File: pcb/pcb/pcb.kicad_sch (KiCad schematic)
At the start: 12 parts, among them J1 SD Card, J2 Mic, J3 Relay Solenoid, J4 Status LED, SW1 Button Up, SW2 Button Down, SW3 Button Record, SW4 Button Delete, SW5 Button Play, U1 ESP32-C3-DevKitC-02

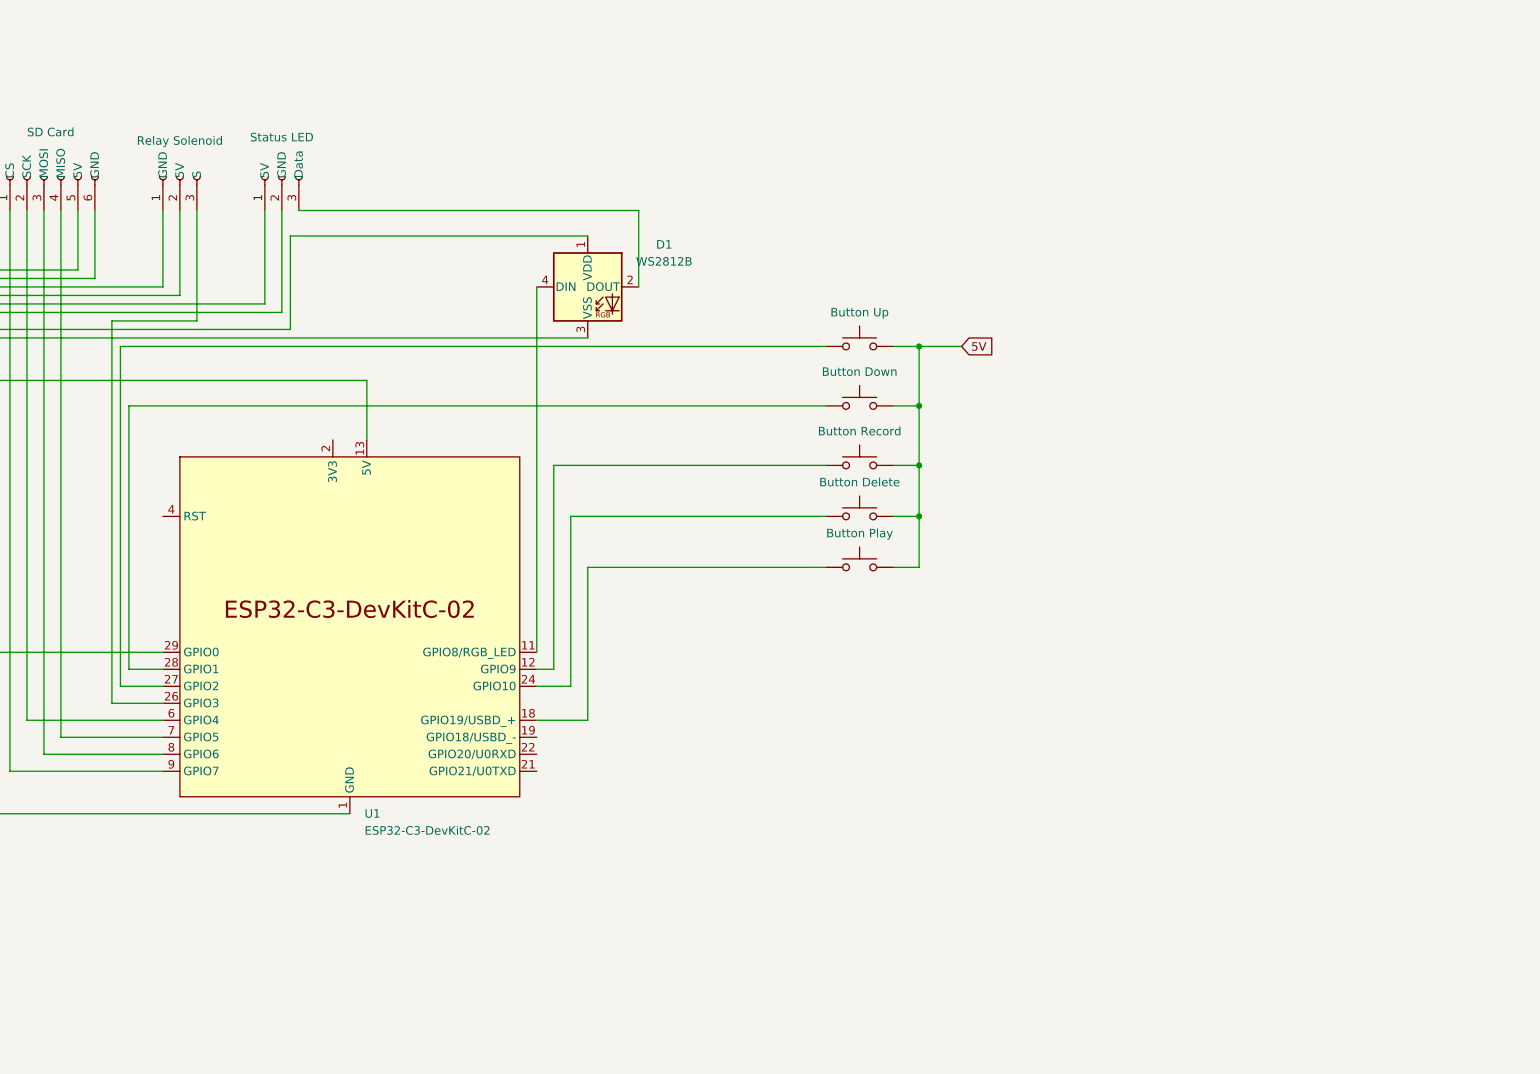
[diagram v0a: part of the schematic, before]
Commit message: update
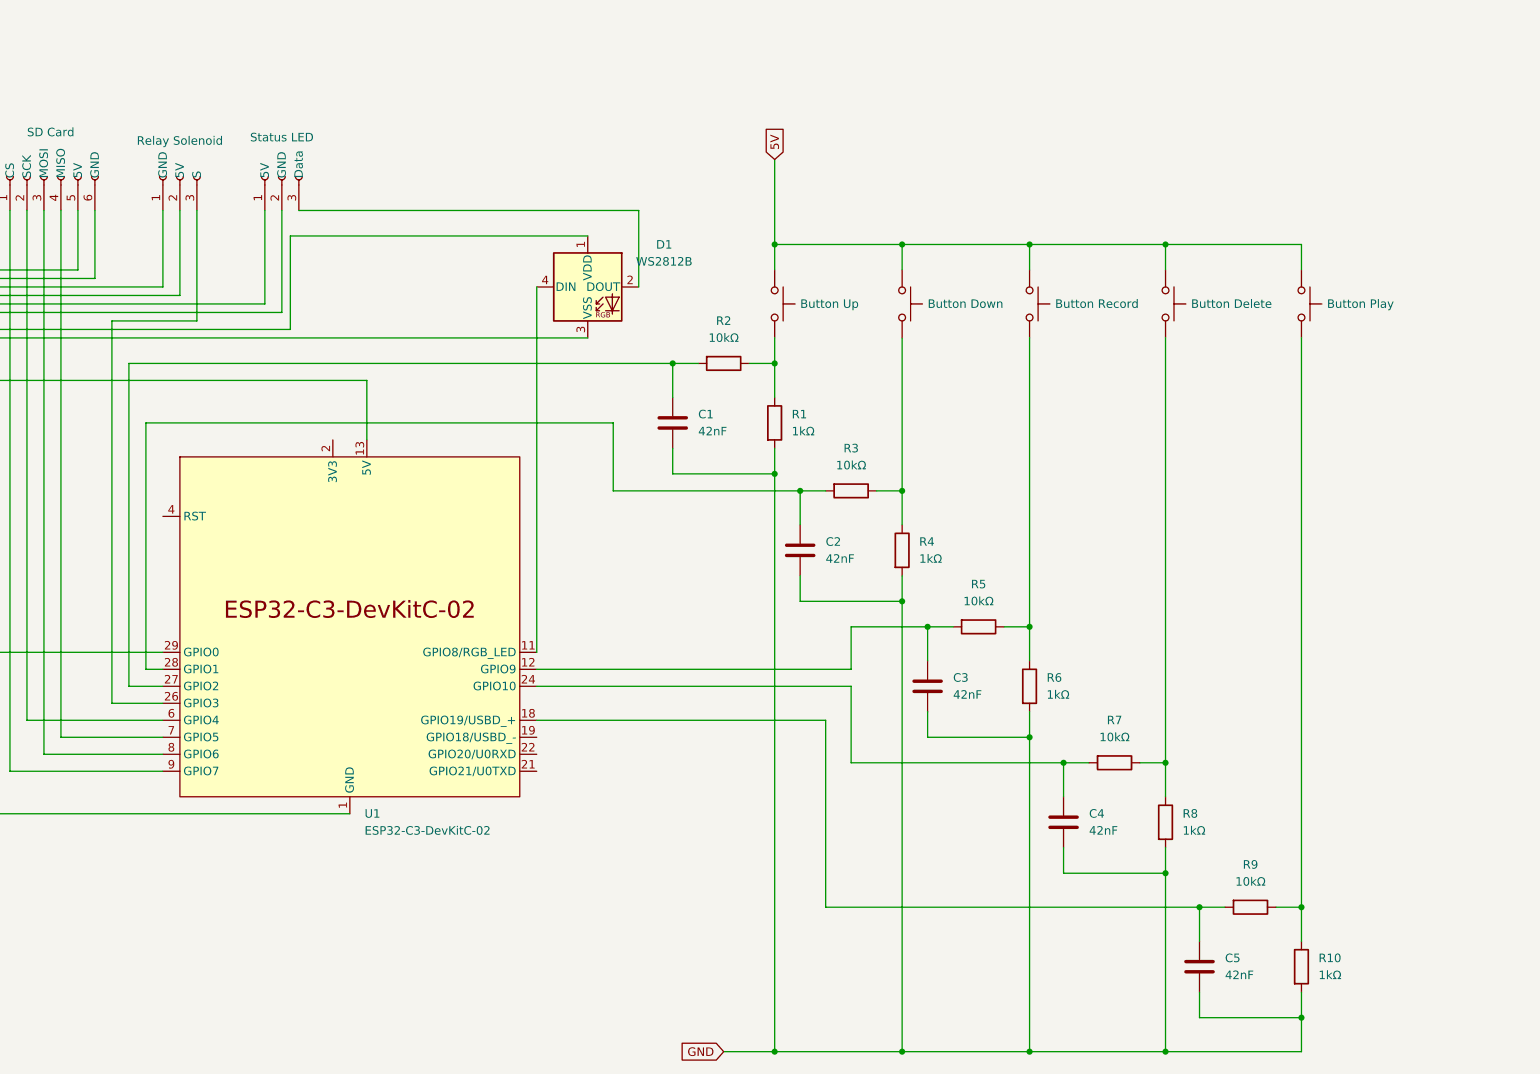
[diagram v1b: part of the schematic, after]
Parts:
- added C1, C2, C3, C4, C5: 42nF, symbol Device:C
- added R1, R10, R4, R6, R8: 1kΩ, symbol Device:R
- added R2, R3, R5, R7, R9: 10kΩ, symbol Device:R
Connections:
- net 5V: now also SW1.1, SW2.1, SW3.1, SW4.1, SW5.1; no longer SW1.2, SW2.2, SW3.2, SW4.2, SW5.2
- net GND: now also C1.2, C2.2, C3.2, C4.2, C5.2, R1.2, R10.2, R4.2, R6.2, R8.2
- net at U1.12 (GPIO9): now also C3.1, R5.2; no longer SW3.1
- net at U1.18 (GPIO19/USBD_+): now also C5.1, R9.2; no longer SW5.1
- net at U1.24 (GPIO10): now also C4.1, R7.2; no longer SW4.1
- net at U1.27 (GPIO2): now also C1.1, R2.2; no longer SW1.1
- net at U1.28 (GPIO1): now also C2.1, R3.2; no longer SW2.1
- new net: R7.1, R8.1, SW4.2
- new net: R1.1, R2.1, SW1.2
- new net: R10.1, R9.1, SW5.2
- new net: R3.1, R4.1, SW2.2
- new net: R5.1, R6.1, SW3.2
